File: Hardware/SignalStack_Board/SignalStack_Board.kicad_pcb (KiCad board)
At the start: 2 copper layers, 92.6 x 80.4 mm, 74 parts, among them J2 RJ45_LED_Shielded, J3 Molex_uF_SV_06, Q1 SI4156DY, Q2 SI4156DY, Q3 SI4156DY, Q4 SI4156DY, Q5 SI4156DY, Q6 SI4156DY, Q7 SI4156DY, Q8 SI4156DY, Q9 Q_PMOS_DGS, SW1 SW_Push, SW2 SW_Push, U1 OKI, U10 74LVC2G04, U2 SMAJ12CA, U3 Teensy4.1_DEV-16771, U4 TSR_1-2450, U5 IRS2005S, U6 IRS2005S, U7 74LVC2G04, U8 IRS2005S, U9 IRS2005S

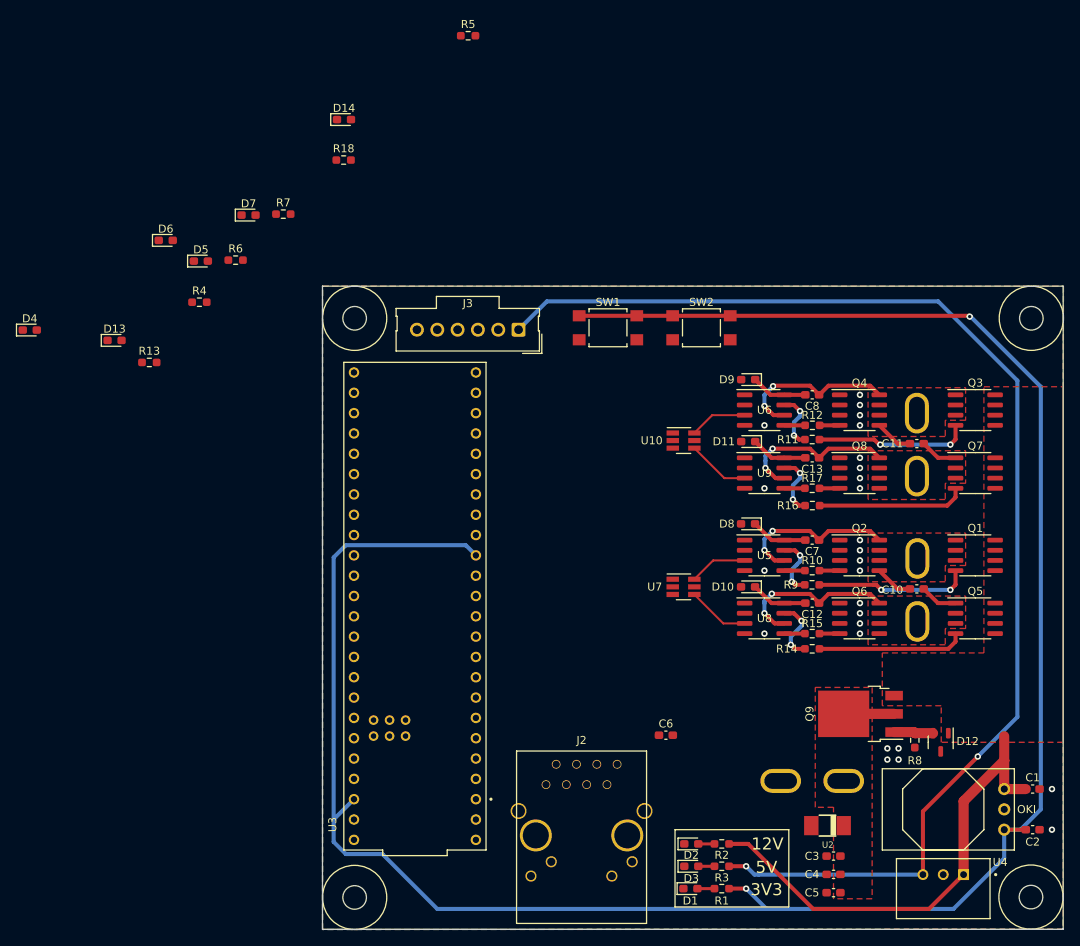
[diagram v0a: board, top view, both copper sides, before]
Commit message: Finished layout
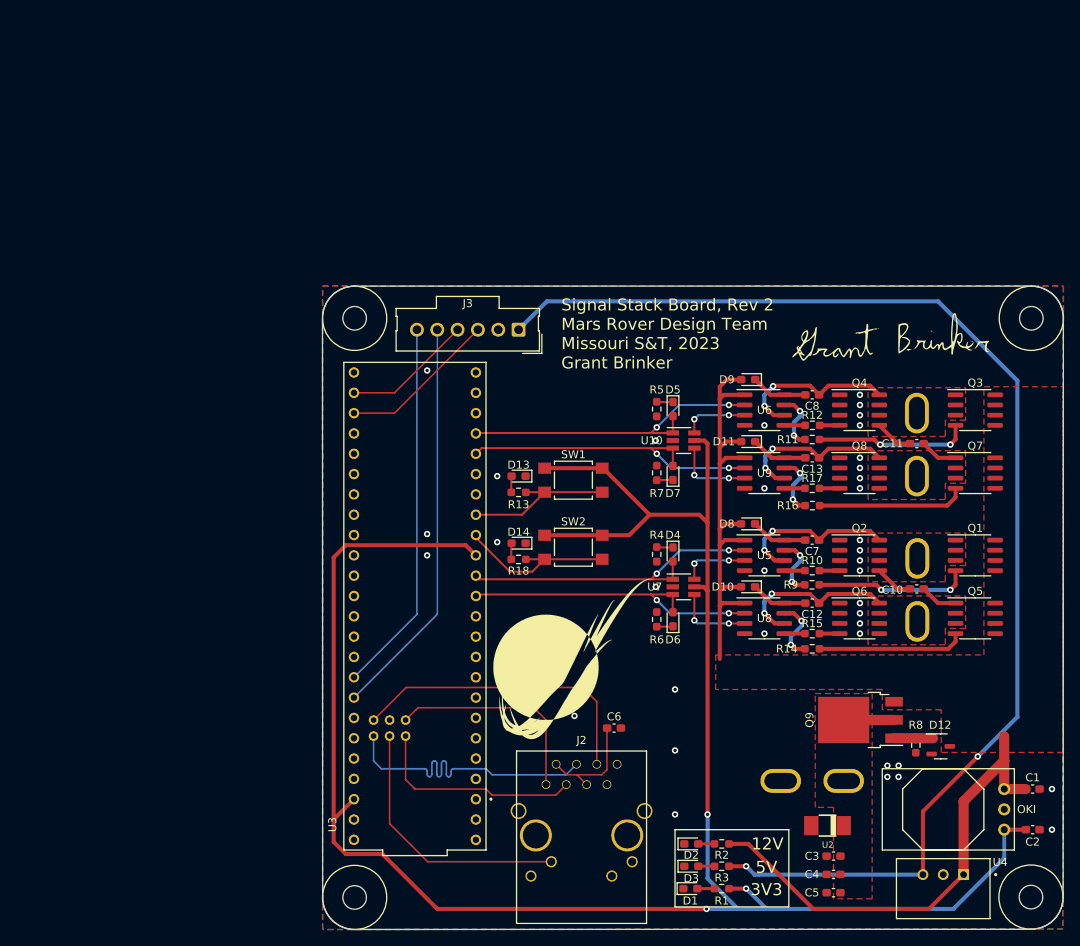
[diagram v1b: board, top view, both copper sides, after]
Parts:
- added G***: LOGO, MRDT_Silkscreens:0_MRDT_Logo_20mm, F.Cu at (143.8, 104.6)
- added G***: LOGO, MRDT_Silkscreens:z_sig_Grant_Brinker_25mmx6, F.Cu at (183.6, 64.5)
- moved D4 85.2 mm to (156.2, 91.6), turned to -90 degrees
- moved D6 79.1 mm to (156.2, 99.7), turned to 90 degrees
- moved R6 69.2 mm to (154.2, 99.7), turned to -90 degrees
- moved R4 65.3 mm to (154.2, 91.6), turned to 90 degrees
- moved D7 62.1 mm to (156.2, 81.4), turned to 90 degrees
- moved D5 61.8 mm to (156.2, 73.4), turned to -90 degrees
- moved D14 57.3 mm to (136.9, 90.2), turned to 180 degrees
- moved R7 56.8 mm to (154.2, 81.4), turned to -90 degrees
- moved R18 54.5 mm to (136.9, 92.2), turned to 180 degrees
- moved D13 53.3 mm to (136.9, 81.8), turned to 180 degrees
- moved R5 52.3 mm to (154.2, 73.4), turned to 90 degrees
- moved R13 48.9 mm to (136.9, 83.8), turned to 180 degrees
- moved SW2 31.8 mm to (143.8, 90.7)
- moved SW1 19.5 mm to (143.8, 82.3)
- moved C6 6.54 mm to (148.8, 113.3)
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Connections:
- U3 pad 0: GPS RX -> unconnected-(U3-Pad0)
- U3 pad 1: GPS TX -> unconnected-(U3-Pad1)
- U3 pad 11: unconnected-(U3-Pad11) -> Coil1_RVS
- U3 pad 12: unconnected-(U3-Pad12) -> Coil1_FWD
- U3 pad 14: Coil1_FWD -> unconnected-(U3-Pad14)
- U3 pad 15: Coil1_RVS -> unconnected-(U3-Pad15)
- U3 pad 22: Coil2_FWD -> unconnected-(U3-Pad22)
- U3 pad 23: Coil2_RVS -> unconnected-(U3-Pad23)
- U3 pad 28: unconnected-(U3-Pad28) -> Coil2_RVS
- U3 pad 29: unconnected-(U3-Pad29) -> Coil2_FWD
- U3 pad 34: unconnected-(U3-Pad34) -> GPS RX
- U3 pad 35: unconnected-(U3-Pad35) -> GPS TX
- U3 pad R-: (no net) -> /RX-
- U3 pad T-: (no net) -> /TX-
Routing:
- net +12V: track 60.1 -> 119.3 mm
- net I2C SCL: track 0.00 -> 50.3 mm
- net I2C SDA: track 0.00 -> 46.7 mm
- net Coil1_FWD: track 0.00 -> 40.5 mm, vias 0 -> 2
- net Coil2_FWD: track 0.00 -> 40.0 mm, vias 0 -> 2
- net Coil2_RVS: track 0.00 -> 40.0 mm, vias 0 -> 2
- net Coil1_RVS: track 0.00 -> 39.6 mm, vias 0 -> 2
- net /RX-: track 0.00 -> 38.2 mm
- net /RX+: track 0.00 -> 38.0 mm
- net /LED: track 0.00 -> 33.1 mm
- net /TX+: track 0.00 -> 26.9 mm
- net /TX-: track 0.00 -> 26.9 mm
- net Motor 1: track 0.00 -> 20.9 mm
- net GPS TX: track 0.00 -> 19.8 mm
- net Motor 2: track 0.00 -> 19.3 mm
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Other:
- outline, holes or cut-outs redrawn
- board text added: "Signal Stack Board, Rev 2 Mars Rover Design Team Missouri S&T, 2023 Grant Brinker"
